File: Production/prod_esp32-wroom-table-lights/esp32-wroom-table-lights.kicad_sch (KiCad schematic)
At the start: 6 parts, among them J1 I2C, U4 ESP32-C3 SuperMini

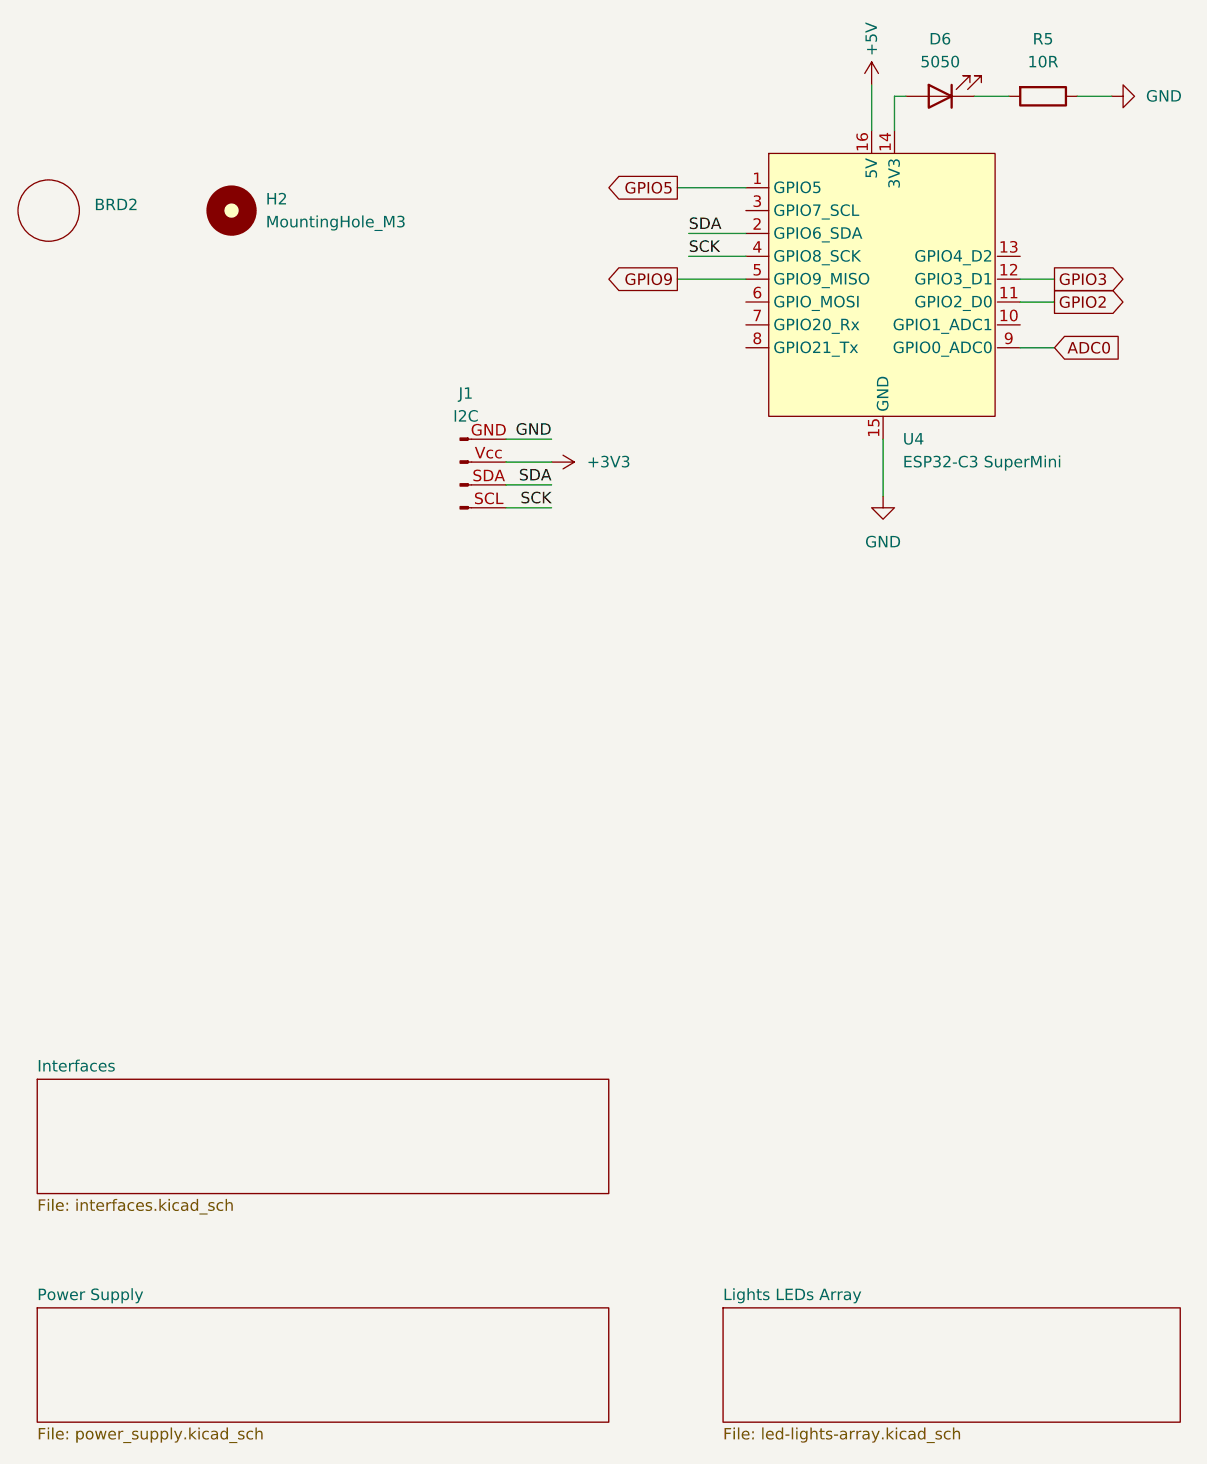
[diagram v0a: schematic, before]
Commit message: .
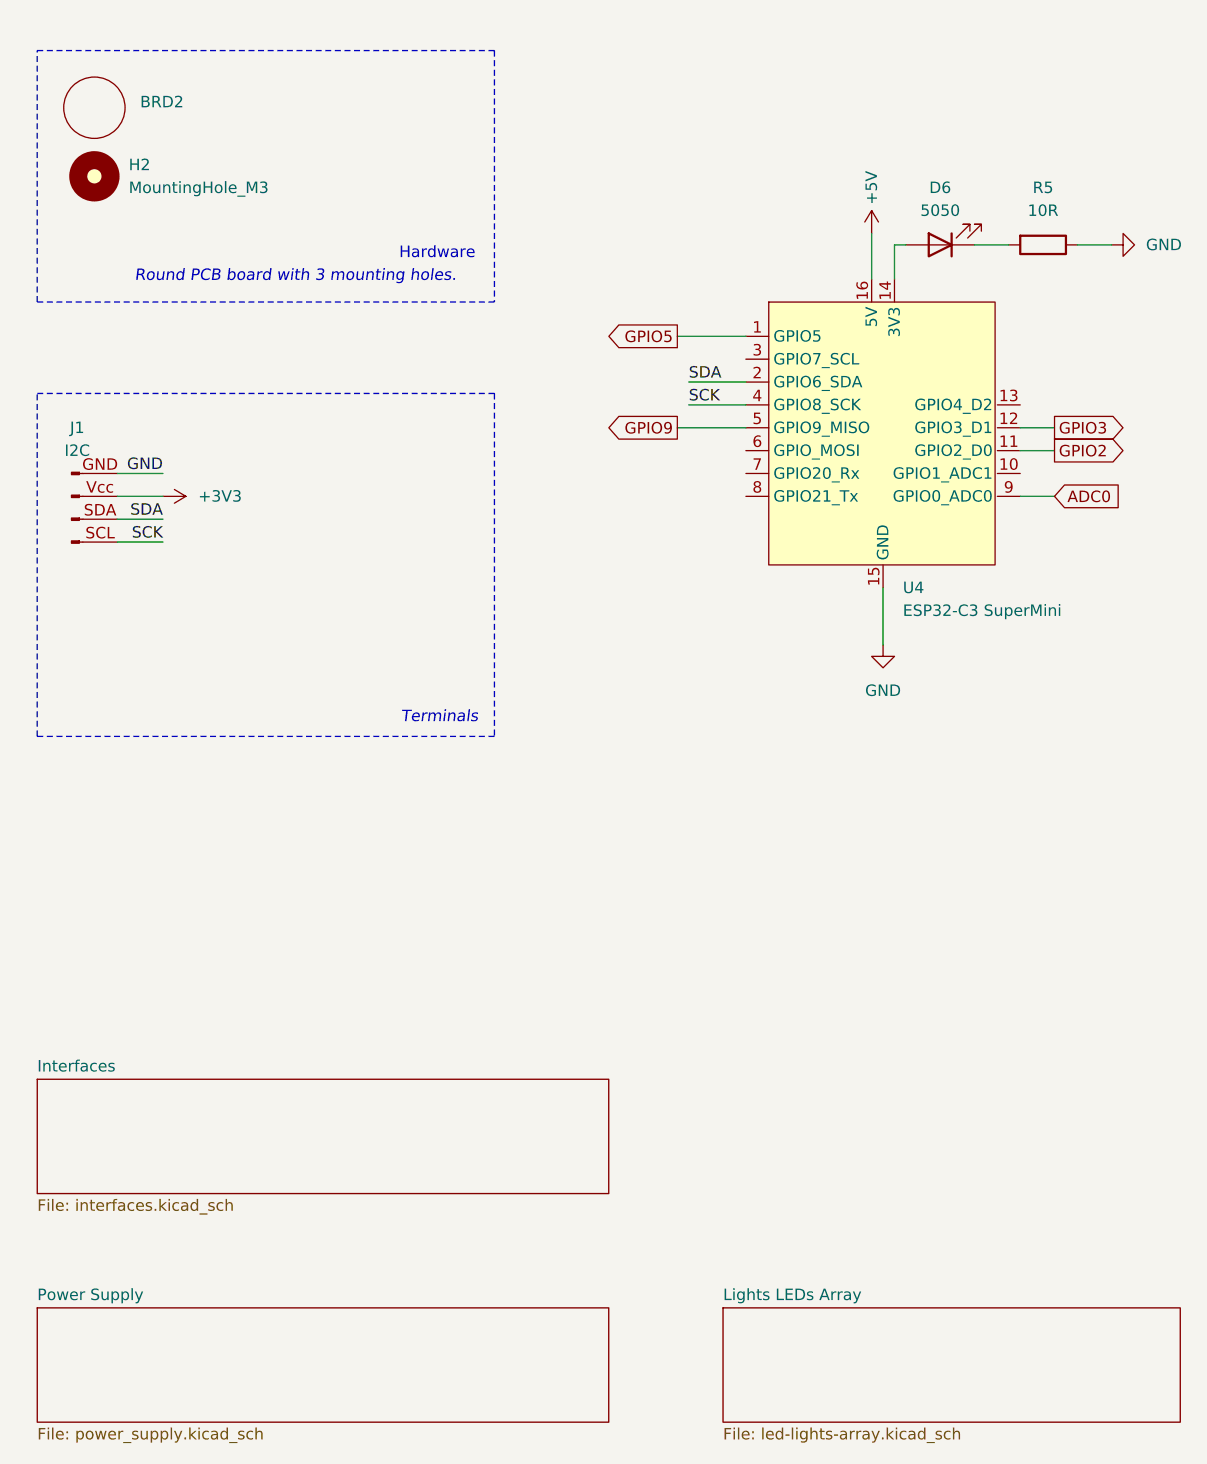
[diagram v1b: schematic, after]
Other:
- note added: "Hardware"
- note added: "Round PCB board with 3 mounting holes."
- note added: "Terminals"
- moved on the sheet: BRD2, D6, H2, J1, R5, U4
